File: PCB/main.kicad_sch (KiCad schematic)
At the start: 59 parts, among them J1 S20B-PADSS-1, J2 S20B-PADSS-1, J3 SWD, SW1 SPST, U1 TPS54302, U2 XC6206P33, U3 TJA1051T/3, U4 TJA1051T/3, U5 STM32G0B1, Y1 ${Frequency}

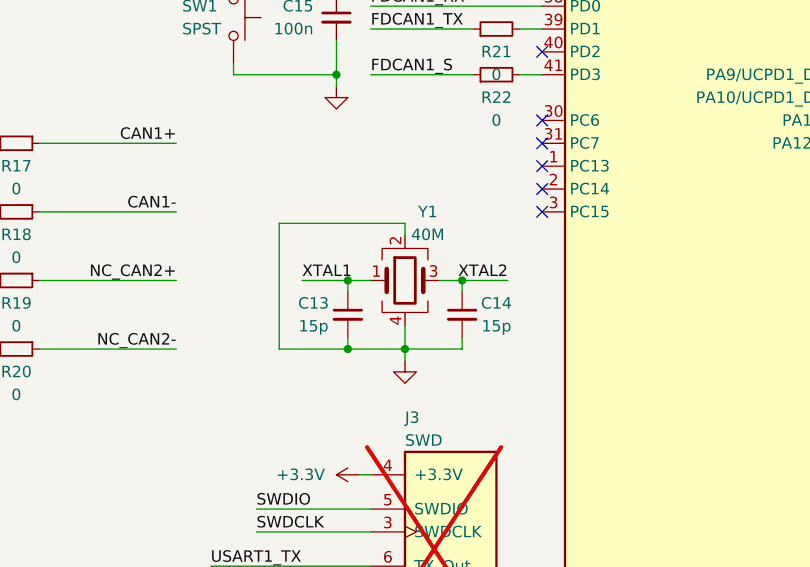
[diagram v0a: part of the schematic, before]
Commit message: Generate output files
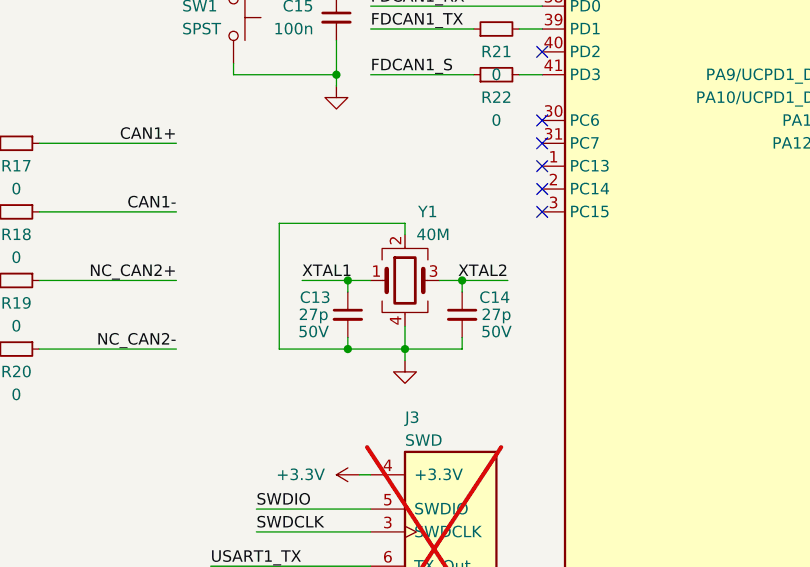
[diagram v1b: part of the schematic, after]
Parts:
- C13, C14: symbol 0 Passive_Components:Capacitors/CMP-0005 -> 0 Passive_Components:Capacitors/CMP-0072; Capacitance 15p -> 27p; LCSC C1548 -> C1557; MPN 0402CG150J500NT -> 0402CG270J500NT
- Y1: footprint libdb:CMP-0004 -> Crystal:Crystal_SMD_3225-4Pin_3.2x2.5mm; symbol 0 Passive_Components:Crystals/CMP-0004 -> 0 Passive_Components:Crystals/CMP-0071; LCSC C485379 -> C9010; Load Capacitance 8p -> 15p; MPN NX2016SA-40M-STD-CZS-3 -> X322540MPB4SI; Manufacturer NDK -> Yangxing Tech
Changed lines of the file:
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@@
   (junction (at 49.53 74.295) (diameter 0) (color 0 0 0 0)
   )
-  (junction (at 200.66 114.3) (diameter 0) (color 0 0 0 0)
-  )
   (junction (at 242.57 48.26) (diameter 0) (color 0 0 0 0)
   )
@@
   (junction (at 143.51 59.055) (diameter 0) (color 0 0 0 0)
   )
+  (junction (at 200.66 114.3) (diameter 0) (color 0 0 0 0)
+  )
   (junction (at 199.39 71.12) (diameter 0) (color 0 0 0 0)
   )
@@
     (stroke (width 0) (type default))
   )
+  (wire (pts (xy 200.66 114.3) (xy 207.01 114.3))
+    (stroke (width 0) (type default))
+  )
   (wire (pts (xy 45.72 186.69) (xy 59.69 186.69))
     (stroke (width 0) (type default))
@@
     (stroke (width 0) (type default))
   )
-  (wire (pts (xy 200.66 114.3) (xy 207.01 114.3))
-    (stroke (width 0) (type default))
-  )
   (wire (pts (xy 266.7 124.46) (xy 278.13 124.46))
     (stroke (width 0) (type default))
@@
     (stroke (width 0) (type default))
   )
-  (wire (pts (xy 200.66 113.03) (xy 200.66 114.3))
-    (stroke (width 0) (type default))
-  )
   (wire (pts (xy 260.35 96.52) (xy 278.13 96.52))
     (stroke (width 0) (type default))
@@
     (stroke (width 0) (type default))
   )
+  (wire (pts (xy 200.66 113.03) (xy 200.66 114.3))
+    (stroke (width 0) (type default))
+  )
   (wire (pts (xy 45.72 148.59) (xy 59.69 148.59))
     (stroke (width 0) (type default))
@@
     )
   )
-  (symbol (lib_id "0 Passive_Components:Crystals/CMP-0004") (at 207.01 106.68 0) (unit 1)
+  (symbol (lib_id "0 Passive_Components:Crystals/CMP-0071") (at 207.01 106.68 0) (unit 1)
     (in_bom yes) (on_board yes) (dnp no)
     (property "Reference" "Y1" (at 209.55 99.06 0)
       (effects (font (size 1.27 1.27)))
     )
-    (property "Value" "${Frequency}" (at 209.55 101.6 0)
-      (effects (font (size 1.27 1.27)))
+    (property "Value" "${Frequency}" (at 208.28 101.6 0)
+      (effects (font (size 1.27 1.27)) (justify left))
     )
-    (property "Footprint" "libdb:CMP-0004" (at 207.01 106.68 0)
+    (property "Footprint" "Crystal:Crystal_SMD_3225-4Pin_3.2x2.5mm" (at 207.01 106.68 0)
       (effects (font (size 1.27 1.27)) hide)
     )
@@
       (effects (font (size 1.27 1.27)) hide)
     )
-    (property "Manufacturer" "NDK " (at 207.01 106.68 0)
+    (property "Manufacturer" "Yangxing Tech" (at 207.01 106.68 0)
       (effects (font (size 1.27 1.27)) hide)
     )
-    (property "MPN" "NX2016SA-40M-STD-CZS-3" (at 207.01 106.68 0)
+    (property "MPN" "X322540MPB4SI" (at 207.01 106.68 0)
       (effects (font (size 1.27 1.27)) hide)
     )
@@
       (effects (font (size 1.27 1.27)) hide)
     )
-    (property "Load Capacitance" "8p" (at 207.01 106.68 0)
+    (property "Load Capacitance" "15p" (at 207.01 106.68 0)
       (effects (font (size 1.27 1.27)) hide)
     )
@@
       (effects (font (size 1.27 1.27)) hide)
     )
-    (property "LCSC" "C485379" (at 207.01 106.68 0) (show_name)
+    (property "LCSC" "C9010" (at 207.01 106.68 0) (show_name)
       (effects (font (size 1.27 1.27)) hide)
     )
@@
     )
   )
-  (symbol (lib_id "0 Passive_Components:Capacitors/CMP-0005") (at 200.66 110.49 0) (mirror y) (unit 1)
+  (symbol (lib_id "0 Passive_Components:Capacitors/CMP-0072") (at 200.66 110.49 0) (mirror y) (unit 1)
     (in_bom yes) (on_board yes) (dnp no)
-    (property "Reference" "C13" (at 196.85 109.22 0)
-      (effects (font (size 1.27 1.27)))
+    (property "Reference" "C13" (at 198.755 108.585 0)
+      (effects (font (size 1.27 1.27)) (justify left))
     )
-    (property "Value" "${Capacitance}" (at 196.85 111.76 0)
+    (property "Value" "${Capacitance}" (at 196.85 110.49 0)
       (effects (font (size 1.27 1.27)))
     )
@@
       (effects (font (size 1.27 1.27)) hide)
     )
-    (property "MPN" "0402CG150J500NT" (at 200.66 110.49 0)
+    (property "MPN" "0402CG270J500NT" (at 200.66 110.49 0)
       (effects (font (size 1.27 1.27)) hide)
     )
-    (property "Capacitance" "15p" (at 200.66 110.49 0)
+    (property "Capacitance" "27p" (at 200.66 110.49 0)
       (effects (font (size 1.27 1.27)) hide)
     )
-    (property "Capacitance Tolerance" "5%" (at 191.77 110.49 90)
+    (property "Capacitance Tolerance" "5%" (at 200.66 110.49 0)
       (effects (font (size 1.27 1.27)) hide)
     )
-    (property "Voltage Rating" "50V" (at 191.77 110.49 90)
-      (effects (font (size 1.27 1.27)) hide)
+    (property "Voltage Rating" "50V" (at 196.85 112.395 0)
+      (effects (font (size 1.27 1.27)))
     )
     (property "Dielectric" "C0G" (at 200.66 110.49 0)
       (effects (font (size 1.27 1.27)) hide)
     )
-    (property "Case Package Size" "0402" (at 186.69 110.49 90)
+    (property "Case Package Size" "0402" (at 200.66 110.49 0)
       (effects (font (size 1.27 1.27)) hide)
     )
-    (property "LCSC" "C1548" (at 200.66 110.49 0) (show_name)
+    (property "LCSC" "C1557" (at 200.66 110.49 0) (show_name)
       (effects (font (size 1.27 1.27)) hide)
     )
@@
     )
   )
-  (symbol (lib_id "0 Passive_Components:Capacitors/CMP-0005") (at 213.36 110.49 0) (unit 1)
+  (symbol (lib_id "0 Passive_Components:Capacitors/CMP-0072") (at 213.36 110.49 0) (unit 1)
     (in_bom yes) (on_board yes) (dnp no)
-    (property "Reference" "C14" (at 217.17 109.22 0)
-      (effects (font (size 1.27 1.27)))
+    (property "Reference" "C14" (at 215.265 108.585 0)
+      (effects (font (size 1.27 1.27)) (justify left))
     )
-    (property "Value" "${Capacitance}" (at 217.17 111.76 0)
+    (property "Value" "${Capacitance}" (at 217.17 110.49 0)
       (effects (font (size 1.27 1.27)))
     )
@@
       (effects (font (size 1.27 1.27)) hide)
     )
-    (property "MPN" "0402CG150J500NT" (at 213.36 110.49 0)
+    (property "MPN" "0402CG270J500NT" (at 213.36 110.49 0)
       (effects (font (size 1.27 1.27)) hide)
     )
-    (property "Capacitance" "15p" (at 213.36 110.49 0)
+    (property "Capacitance" "27p" (at 213.36 110.49 0)
       (effects (font (size 1.27 1.27)) hide)
     )
-    (property "Capacitance Tolerance" "5%" (at 222.25 110.49 90)
+    (property "Capacitance Tolerance" "5%" (at 213.36 110.49 0)
       (effects (font (size 1.27 1.27)) hide)
     )
-    (property "Voltage Rating" "50V" (at 217.17 110.49 90)
-      (effects (font (size 1.27 1.27)) hide)
+    (property "Voltage Rating" "50V" (at 217.17 112.395 0)
+      (effects (font (size 1.27 1.27)))
     )
     (property "Dielectric" "C0G" (at 213.36 110.49 0)
       (effects (font (size 1.27 1.27)) hide)
     )
-    (property "Case Package Size" "0402" (at 217.17 110.49 90)
+    (property "Case Package Size" "0402" (at 213.36 110.49 0)
       (effects (font (size 1.27 1.27)) hide)
     )
-    (property "LCSC" "C1548" (at 213.36 110.49 0) (show_name)
+    (property "LCSC" "C1557" (at 213.36 110.49 0) (show_name)
       (effects (font (size 1.27 1.27)) hide)
     )
